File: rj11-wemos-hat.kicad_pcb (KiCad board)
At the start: 2 copper layers, 39.3 x 46.5 mm, 25 parts, among them J0 Conn_02x12_Odd_Even, J1 RJ10, J10 SDA, J11 D6, J12 D5, J13 D7, J14 D8, J15 D0, J16 D4, J2 RJ10, J6 D3, J7 TX, J8 RX, J9 SCL, SW1 RST, SW2 Flash

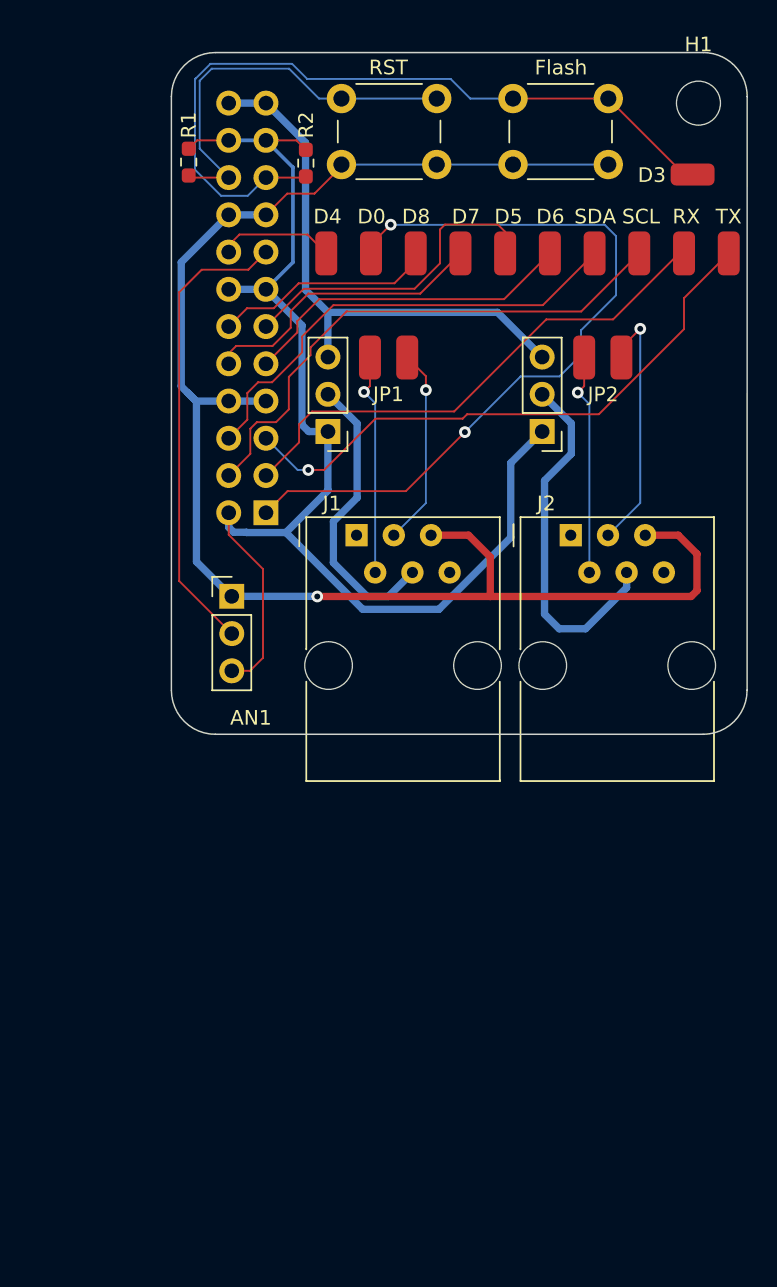
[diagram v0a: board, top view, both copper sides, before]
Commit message: Format changes and first assembly
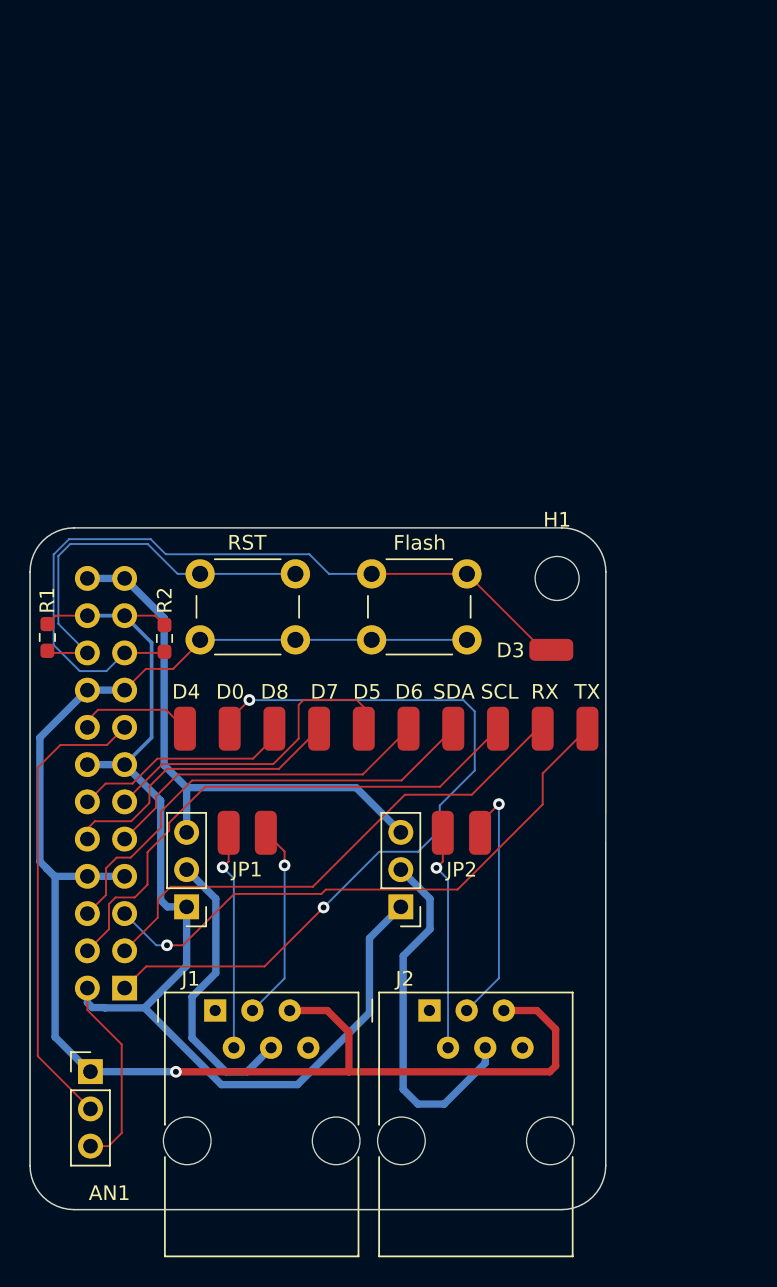
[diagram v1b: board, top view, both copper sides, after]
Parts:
- moved J6 33.8 mm to (90.0, 78.0)
- moved AN1 33.8 mm to (58.5, 106.8)
- moved H1 33.8 mm to (90.4, 73.2)
- moved J0 33.8 mm to (60.9, 101.1)
- moved J1 33.8 mm to (67.0, 102.6)
- moved J10 33.8 mm to (83.3, 83.4)
- moved J11 33.8 mm to (80.2, 83.4)
- moved J12 33.8 mm to (77.2, 83.4)
- moved J13 33.8 mm to (74.1, 83.4)
- moved J14 33.8 mm to (71.1, 83.4)
- moved J15 33.8 mm to (68.0, 83.4)
- moved J16 33.8 mm to (65.0, 83.4)
- moved J2 33.8 mm to (81.7, 102.6)
- moved J7 33.8 mm to (92.4, 83.4)
- moved J8 33.8 mm to (89.4, 83.4)
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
